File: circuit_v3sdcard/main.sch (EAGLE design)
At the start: 20 parts, among them CN1 SD, CN3 MICROSD, CN4 5035481020, IC1 C8051F381-GM, IC3 N25Q512A, IC4 KC2016K, IC6 MPU-9250

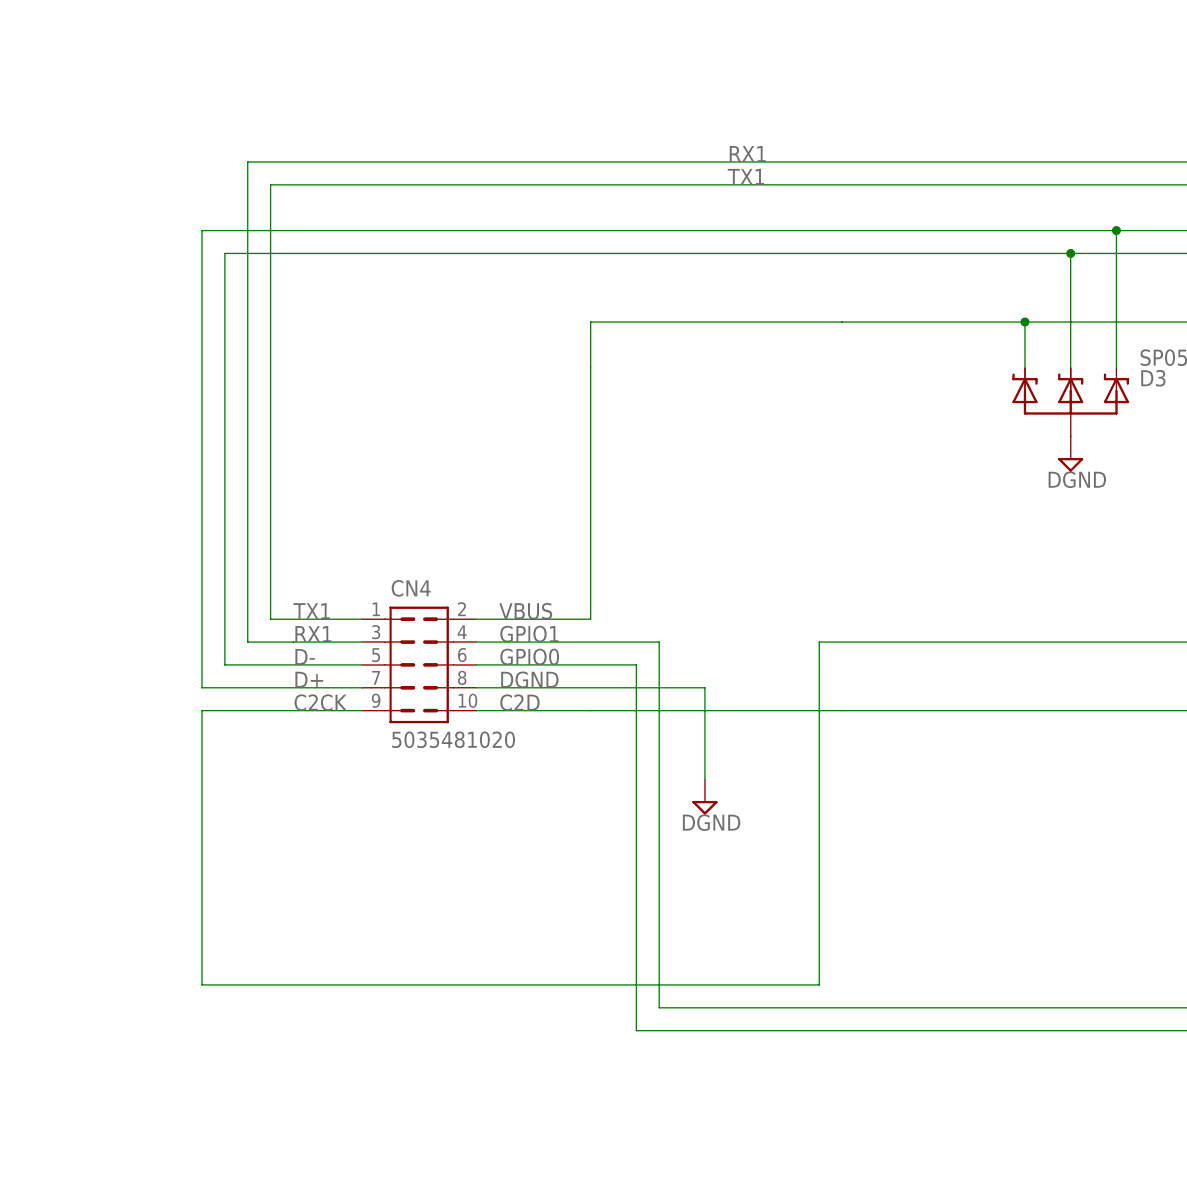
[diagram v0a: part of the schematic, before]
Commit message: Modified circuit
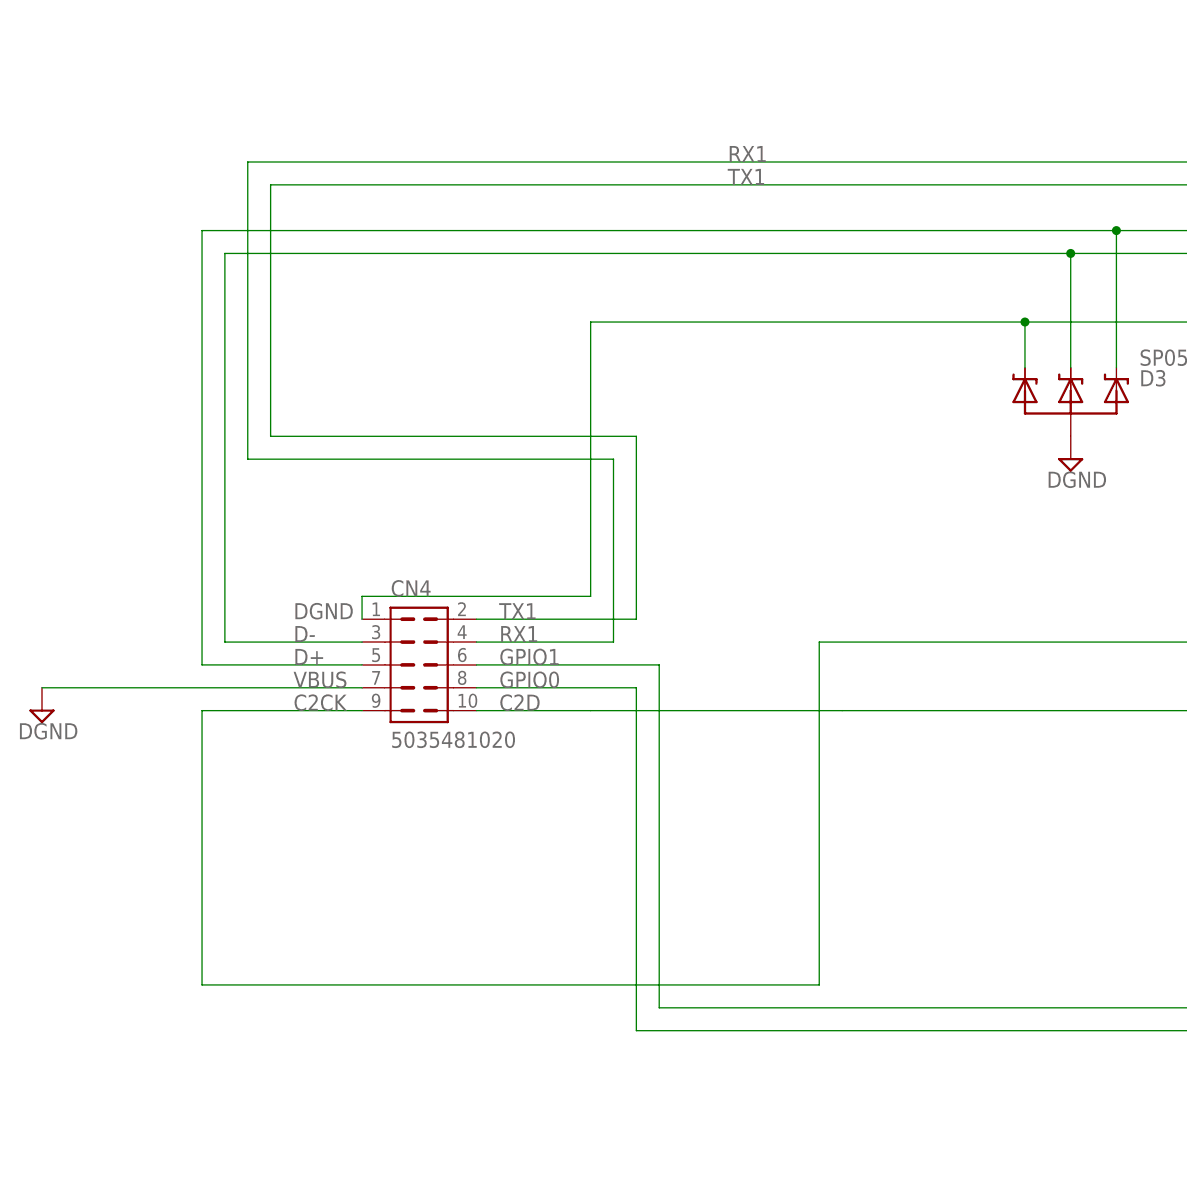
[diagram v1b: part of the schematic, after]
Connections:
- net D+: now also CN4.5; no longer CN4.7
- net D-: now also CN4.3; no longer CN4.5
- net DGND: now also CN4.7; no longer CN4.8
- net GPIO0: now also CN4.8; no longer CN4.6
- net GPIO1: now also CN4.6; no longer CN4.4
- net RX1: now also CN4.4; no longer CN4.3
- net TX1: now also CN4.2; no longer CN4.1
- net VBUS: now also CN4.1; no longer CN4.2
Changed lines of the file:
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@@
 <instance part="R1" gate="G$1" x="-55.88" y="-17.78" rot="R90"/>
 <instance part="SUPPLY3" gate="G$1" x="-55.88" y="-22.86"/>
-<instance part="SUPPLY1" gate="G$1" x="-144.78" y="-60.96"/>
+<instance part="SUPPLY1" gate="G$1" x="-218.44" y="-50.8"/>
 <instance part="D4" gate="A" x="-48.26" y="-2.54" rot="MR180"/>
 <instance part="R3" gate="G$1" x="-40.64" y="-7.62" rot="R180"/>
@@
 </segment>
 <segment>
-<pinref part="CN4" gate="G$1" pin="8"/>
-<wire x1="-170.18" y1="-48.26" x2="-144.78" y2="-48.26" width="0.1524" layer="91"/>
-<wire x1="-144.78" y1="-48.26" x2="-144.78" y2="-58.42" width="0.1524" layer="91"/>
 <pinref part="SUPPLY1" gate="G$1" pin="DGND"/>
-<label x="-167.64" y="-48.26" size="1.778" layer="95"/>
+<label x="-190.5" y="-40.64" size="1.778" layer="95"/>
+<pinref part="CN4" gate="G$1" pin="7"/>
+<wire x1="-182.88" y1="-48.26" x2="-218.44" y2="-48.26" width="0.1524" layer="91"/>
 </segment>
 </net>
@@
 <pinref part="IC1" gate="G$1" pin="D-"/>
 <pinref part="D3" gate="G$1" pin="3"/>
-<label x="-190.5" y="-45.72" size="1.778" layer="95"/>
-<wire x1="-198.12" y1="0" x2="-198.12" y2="-45.72" width="0.1524" layer="91"/>
-<pinref part="CN4" gate="G$1" pin="5"/>
-<wire x1="-198.12" y1="-45.72" x2="-182.88" y2="-45.72" width="0.1524" layer="91"/>
+<label x="-190.5" y="-43.18" size="1.778" layer="95"/>
+<wire x1="-198.12" y1="0" x2="-198.12" y2="-43.18" width="0.1524" layer="91"/>
+<pinref part="CN4" gate="G$1" pin="3"/>
+<wire x1="-198.12" y1="-43.18" x2="-182.88" y2="-43.18" width="0.1524" layer="91"/>
 </segment>
 </net>
@@
 <pinref part="IC1" gate="G$1" pin="D+"/>
 <pinref part="D3" gate="G$1" pin="2"/>
-<pinref part="CN4" gate="G$1" pin="7"/>
-<wire x1="-200.66" y1="2.54" x2="-200.66" y2="-48.26" width="0.1524" layer="91"/>
-<wire x1="-200.66" y1="-48.26" x2="-182.88" y2="-48.26" width="0.1524" layer="91"/>
-<label x="-190.5" y="-48.26" size="1.778" layer="95"/>
+<wire x1="-200.66" y1="2.54" x2="-200.66" y2="-45.72" width="0.1524" layer="91"/>
+<label x="-190.5" y="-45.72" size="1.778" layer="95"/>
+<pinref part="CN4" gate="G$1" pin="5"/>
+<wire x1="-200.66" y1="-45.72" x2="-182.88" y2="-45.72" width="0.1524" layer="91"/>
 </segment>
 </net>
@@
 <net name="VBUS" class="1">
 <segment>
-<wire x1="-129.54" y1="-7.62" x2="-157.48" y2="-7.62" width="0.1524" layer="91"/>
-<wire x1="-157.48" y1="-7.62" x2="-157.48" y2="-12.7" width="0.1524" layer="91"/>
-<wire x1="-157.48" y1="-12.7" x2="-157.48" y2="-40.64" width="0.1524" layer="91"/>
-<pinref part="CN4" gate="G$1" pin="2"/>
-<wire x1="-157.48" y1="-40.64" x2="-170.18" y2="-40.64" width="0.1524" layer="91"/>
-<label x="-167.64" y="-40.64" size="1.778" layer="95"/>
+<wire x1="-109.22" y1="-7.62" x2="-157.48" y2="-7.62" width="0.1524" layer="91"/>
+<wire x1="-157.48" y1="-7.62" x2="-157.48" y2="-38.1" width="0.1524" layer="91"/>
+<label x="-190.5" y="-48.26" size="1.778" layer="95"/>
 <pinref part="D3" gate="G$1" pin="4"/>
 <wire x1="-109.22" y1="-7.62" x2="-109.22" y2="-12.7" width="0.1524" layer="91"/>
@@
 <junction x="-55.88" y="-7.62"/>
 <wire x1="-55.88" y1="-7.62" x2="-45.72" y2="-7.62" width="0.1524" layer="91"/>
-<wire x1="-129.54" y1="-7.62" x2="-109.22" y2="-7.62" width="0.1524" layer="91"/>
 <junction x="-109.22" y="-7.62"/>
 <pinref part="R3" gate="G$1" pin="P$2"/>
+<pinref part="CN4" gate="G$1" pin="1"/>
+<wire x1="-182.88" y1="-38.1" x2="-157.48" y2="-38.1" width="0.1524" layer="91"/>
+<wire x1="-182.88" y1="-40.64" x2="-182.88" y2="-38.1" width="0.1524" layer="91"/>
 </segment>
 </net>
@@
 <pinref part="IC1" gate="G$1" pin="P0.1"/>
 <wire x1="-22.86" y1="10.16" x2="-195.58" y2="10.16" width="0.1524" layer="91"/>
-<wire x1="-195.58" y1="10.16" x2="-195.58" y2="-43.18" width="0.1524" layer="91"/>
+<wire x1="-195.58" y1="10.16" x2="-195.58" y2="-22.86" width="0.1524" layer="91"/>
 <label x="-142.24" y="10.16" size="1.778" layer="95"/>
-<pinref part="CN4" gate="G$1" pin="3"/>
-<wire x1="-182.88" y1="-43.18" x2="-190.5" y2="-43.18" width="0.1524" layer="91"/>
-<wire x1="-190.5" y1="-43.18" x2="-195.58" y2="-43.18" width="0.1524" layer="91"/>
-<label x="-190.5" y="-43.18" size="1.778" layer="95"/>
+<label x="-167.64" y="-43.18" size="1.778" layer="95"/>
+<wire x1="-195.58" y1="-22.86" x2="-154.94" y2="-22.86" width="0.1524" layer="91"/>
+<wire x1="-154.94" y1="-22.86" x2="-154.94" y2="-43.18" width="0.1524" layer="91"/>
+<pinref part="CN4" gate="G$1" pin="4"/>
+<wire x1="-154.94" y1="-43.18" x2="-170.18" y2="-43.18" width="0.1524" layer="91"/>
 </segment>
 </net>
@@
 <wire x1="-193.04" y1="7.62" x2="-22.86" y2="7.62" width="0.1524" layer="91"/>
 <label x="-142.24" y="7.62" size="1.778" layer="95"/>
-<pinref part="CN4" gate="G$1" pin="1"/>
-<wire x1="-182.88" y1="-40.64" x2="-193.04" y2="-40.64" width="0.1524" layer="91"/>
-<wire x1="-193.04" y1="-40.64" x2="-193.04" y2="7.62" width="0.1524" layer="91"/>
-<label x="-190.5" y="-40.64" size="1.778" layer="95"/>
+<label x="-167.64" y="-40.64" size="1.778" layer="95"/>
+<wire x1="-193.04" y1="-20.32" x2="-193.04" y2="7.62" width="0.1524" layer="91"/>
+<wire x1="-193.04" y1="-20.32" x2="-152.4" y2="-20.32" width="0.1524" layer="91"/>
+<wire x1="-152.4" y1="-20.32" x2="-152.4" y2="-40.64" width="0.1524" layer="91"/>
+<pinref part="CN4" gate="G$1" pin="2"/>
+<wire x1="-170.18" y1="-40.64" x2="-152.4" y2="-40.64" width="0.1524" layer="91"/>
 </segment>
 </net>
 <net name="GPIO0" class="0">
 <segment>
-<label x="-167.64" y="-45.72" size="1.778" layer="95"/>
+<label x="-167.64" y="-48.26" size="1.778" layer="95"/>
 <pinref part="IC1" gate="G$1" pin="P2.6"/>
 <wire x1="0" y1="-22.86" x2="0" y2="-86.36" width="0.1524" layer="91"/>
 <wire x1="0" y1="-86.36" x2="-152.4" y2="-86.36" width="0.1524" layer="91"/>
-<pinref part="CN4" gate="G$1" pin="6"/>
-<wire x1="-152.4" y1="-86.36" x2="-152.4" y2="-45.72" width="0.1524" layer="91"/>
-<wire x1="-152.4" y1="-45.72" x2="-170.18" y2="-45.72" width="0.1524" layer="91"/>
+<wire x1="-152.4" y1="-86.36" x2="-152.4" y2="-48.26" width="0.1524" layer="91"/>
+<pinref part="CN4" gate="G$1" pin="8"/>
+<wire x1="-170.18" y1="-48.26" x2="-152.4" y2="-48.26" width="0.1524" layer="91"/>
 </segment>
 </net>
 <net name="GPIO1" class="0">
 <segment>
-<label x="-167.64" y="-43.18" size="1.778" layer="95"/>
+<label x="-167.64" y="-45.72" size="1.778" layer="95"/>
 <pinref part="IC1" gate="G$1" pin="P2.7"/>
 <wire x1="-149.86" y1="-83.82" x2="-2.54" y2="-83.82" width="0.1524" layer="91"/>
 <wire x1="-2.54" y1="-83.82" x2="-2.54" y2="-22.86" width="0.1524" layer="91"/>
-<pinref part="CN4" gate="G$1" pin="4"/>
-<wire x1="-149.86" y1="-83.82" x2="-149.86" y2="-43.18" width="0.1524" layer="91"/>
-<wire x1="-149.86" y1="-43.18" x2="-170.18" y2="-43.18" width="0.1524" layer="91"/>
-</segment>
-</net>
+<wire x1="-149.86" y1="-83.82" x2="-149.86" y2="-45.72" width="0.1524" layer="91"/>
+<pinref part="CN4" gate="G$1" pin="6"/>
+<wire x1="-170.18" y1="-45.72" x2="-149.86" y2="-45.72" width="0.1524" layer="91"/>
+</segment>
+</net>
